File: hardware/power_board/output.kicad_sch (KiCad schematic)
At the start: 15 parts, among them J6 HEATER, K1 BOOST, K2 OFFPEAK, Q1 MMBT3904, Q2 MMBT3904, U6 PC817, U7 PC817

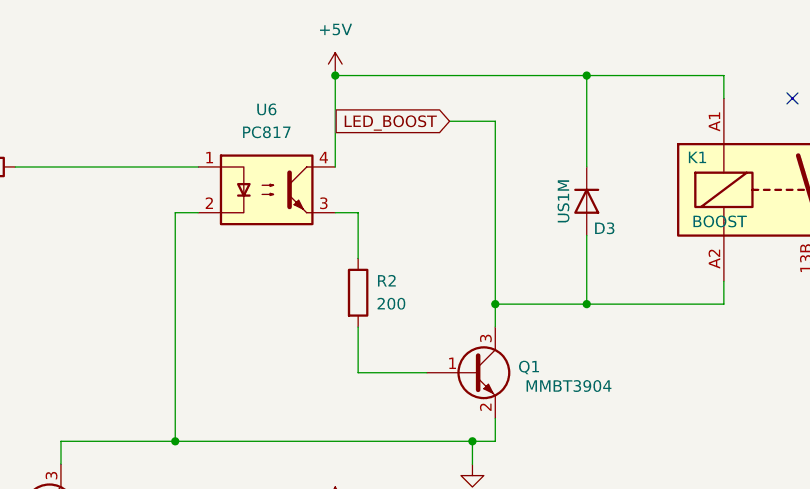
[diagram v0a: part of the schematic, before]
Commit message: v3 first draft
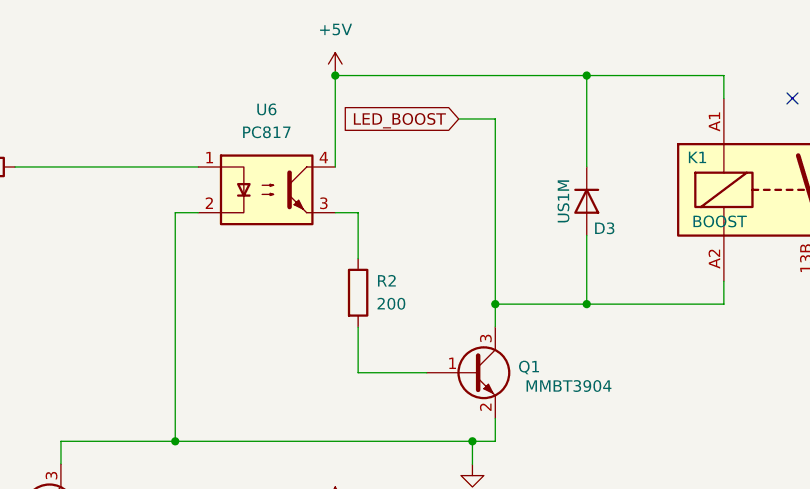
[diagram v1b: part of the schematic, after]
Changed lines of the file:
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@@
     (stroke (width 0) (type default))
   )
-  (wire (pts (xy 129.54 48.26) (xy 129.54 68.58))
+  (wire (pts (xy 129.54 48.006) (xy 129.54 68.58))
     (stroke (width 0) (type default))
   )
@@
     (stroke (width 0) (type default))
   )
-  (wire (pts (xy 124.46 48.26) (xy 129.54 48.26))
+  (wire (pts (xy 125.476 48.006) (xy 129.54 48.006))
     (stroke (width 0) (type default))
   )
@@
     )
   )
-  (global_label "LED_BOOST" (shape input) (at 124.46 48.26 180) (fields_autoplaced)
+  (global_label "LED_BOOST" (shape input) (at 125.476 48.006 180) (fields_autoplaced)
     (effects (font (size 1.27 1.27)) (justify right))
-    (property "Intersheetrefs" "${INTERSHEET_REFS}" (at 110.952 48.26 0)
+    (property "Intersheetrefs" "${INTERSHEET_REFS}" (at 111.968 48.006 0)
       (effects (font (size 1.27 1.27)) (justify right) hide)
     )
